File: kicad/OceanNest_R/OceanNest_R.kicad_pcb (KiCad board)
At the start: 2 copper layers, 4.8 x 4.3 mm, 41 parts, among them J21 TRRS_MJ-4PP-9, J22 Conn_01x07_Pin, SW21 SW_Push, SW22 SW_Push, SW23 SW_Push, SW24 SW_Push, SW25 SW_Push, SW26 SW_Push, SW27 SW_Push, SW28 SW_Push, SW29 SW_Push, SW30 SW_Push, SW31 SW_Push, SW32 SW_Push, SW33 SW_Push, SW34 SW_Push, U21 XIAO-RP2040-DIP

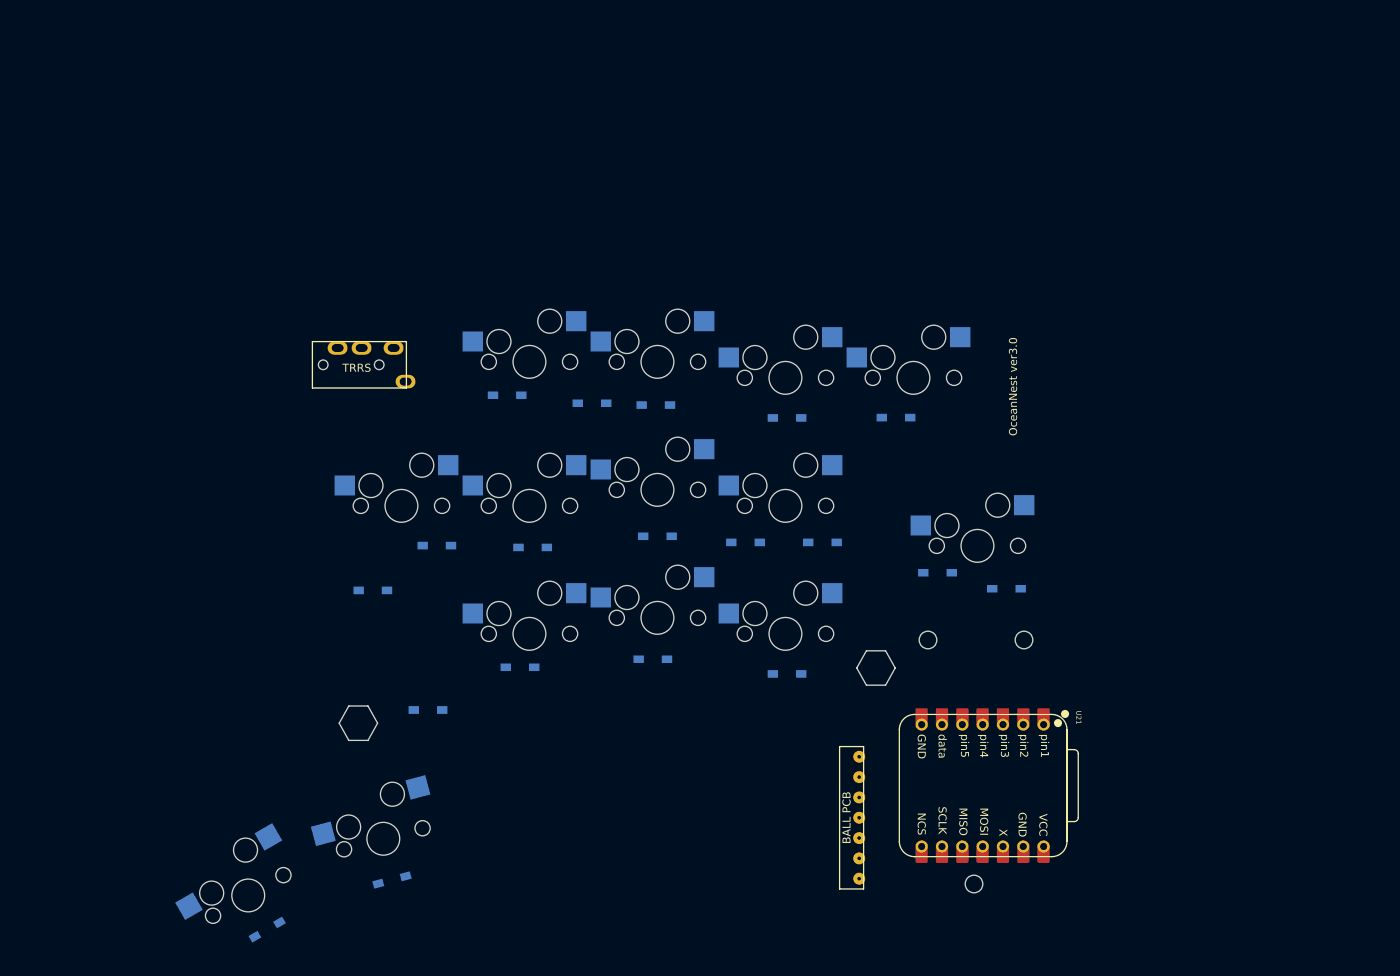
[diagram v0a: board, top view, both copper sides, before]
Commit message: routing
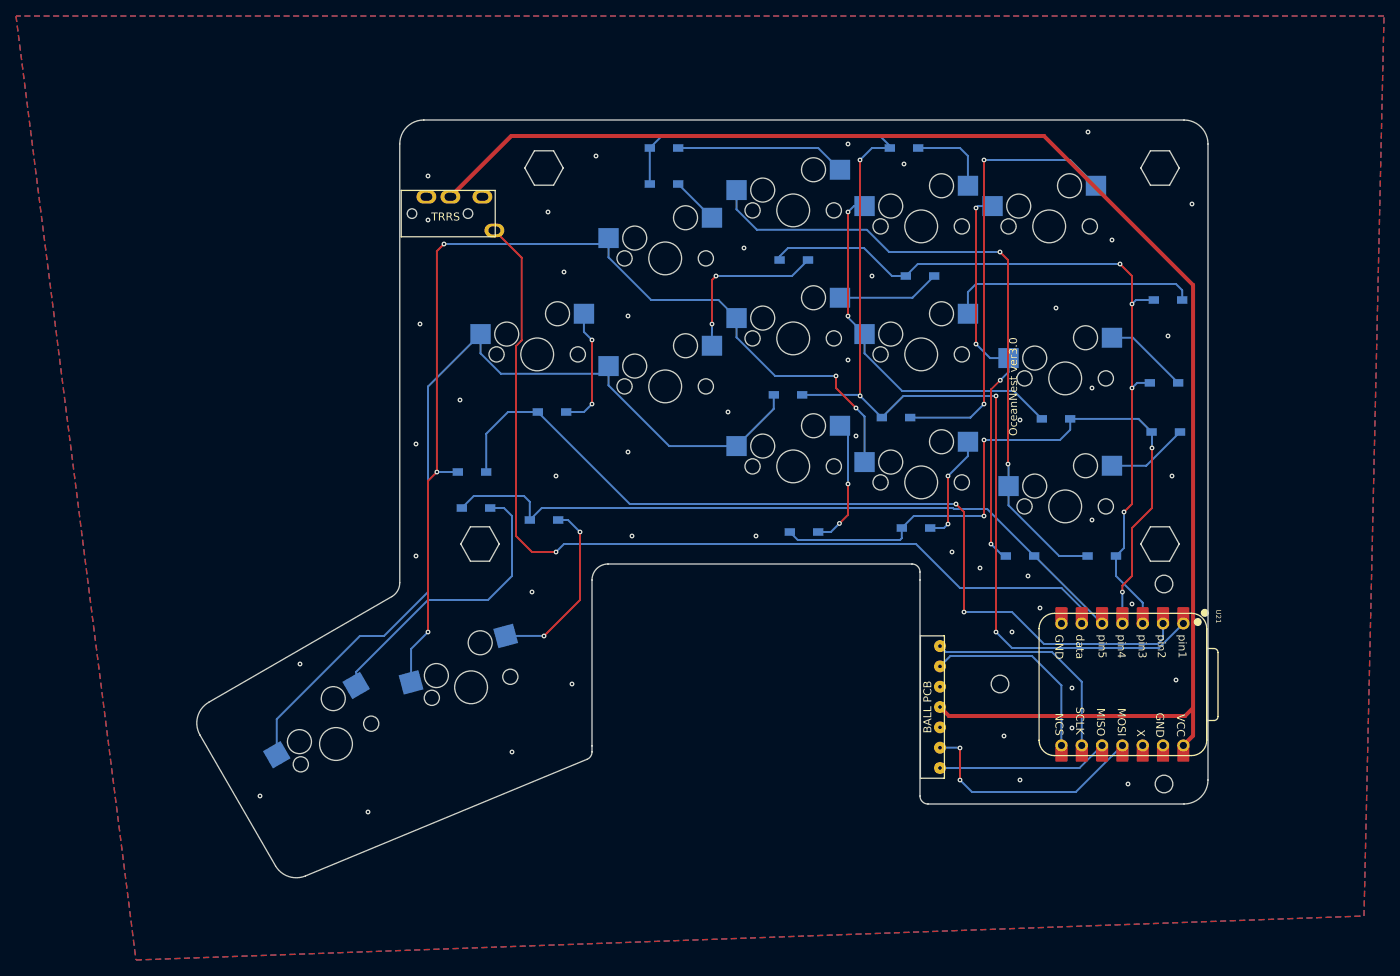
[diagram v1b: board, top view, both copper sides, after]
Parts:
- added hole1: Val**, kbd_Hole:m2_Spacer_Hole_hex, F.Cu at (115.0, 95.0)
- added hole2: Val**, kbd_Hole:m2_Spacer_Hole_hex, F.Cu at (123.0, 48.0)
- moved hole1 102.7 mm to (200.0, 95.0)
- moved D39 76.5 mm to (182.5, 96.5)
- moved hole2 71.9 mm to (200.0, 48.0)
- moved D37 58.8 mm to (114.5, 90.5), turned to 0 degrees
- moved D35 56.2 mm to (200.7, 81.0)
- moved D31 52.8 mm to (201.0, 64.5)
- moved D38 48.8 mm to (123.0, 92.0), turned to 0 degrees
- moved D28 48.5 mm to (154.2, 59.5)
- moved D29 46.2 mm to (170.0, 61.5)
- moved D30 44.6 mm to (192.7, 96.5)
- moved D33 39.3 mm to (155.5, 93.5)
- moved SW30 39.1 mm to (154.2, 85.3)
- moved SW32 38.4 mm to (188.2, 90.3)
- moved SW31 37.1 mm to (170.2, 87.3)
- moved D24 36.8 mm to (168.0, 45.5)
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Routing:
- net VCC: track 0.00 -> 194.3 mm
- net pin1: track 0.00 -> 151.3 mm, vias 0 -> 4
- net Net-(D27-K): track 0.00 -> 130.6 mm, vias 0 -> 5
- net data: track 0.00 -> 117.1 mm, vias 0 -> 1
- net Net-(D21-K): track 0.00 -> 114.6 mm
- net pin2: track 0.00 -> 112.0 mm, vias 0 -> 2
- net pin3: track 0.00 -> 98.7 mm, vias 0 -> 4
- net pin5: track 0.00 -> 89.8 mm
- net pin4: track 0.00 -> 85.2 mm, vias 0 -> 4
- net Net-(D30-K): track 0.00 -> 82.2 mm, vias 0 -> 2
- net Net-(D25-A): track 0.00 -> 55.8 mm, vias 0 -> 2
- net Net-(D39-K): track 0.00 -> 50.6 mm, vias 0 -> 4
- net Net-(D36-K): track 0.00 -> 46.4 mm, vias 0 -> 2
- net Net-(D37-A): track 0.00 -> 38.0 mm
- net Net-(D31-A): track 0.00 -> 31.5 mm
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- added copper zone on B.Cu, net GND
- added copper zone on F.Cu, net GND
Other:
- board size 4.8 x 4.3 mm -> 126.4 x 94.7 mm
